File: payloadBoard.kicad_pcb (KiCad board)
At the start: 2 copper layers, 20 x 45 mm, 40 parts, among them J1 USB_C_Receptacle_USB2.0_16P, J2 SERVO, J3 2S Battery, U1 nRF52833_QDxx, U2 AT25SF041-SSHB-X, U3 LSM6DSO32, U4 AP63205WU, U5 AP63203WU, Y2 Crystal_GND24

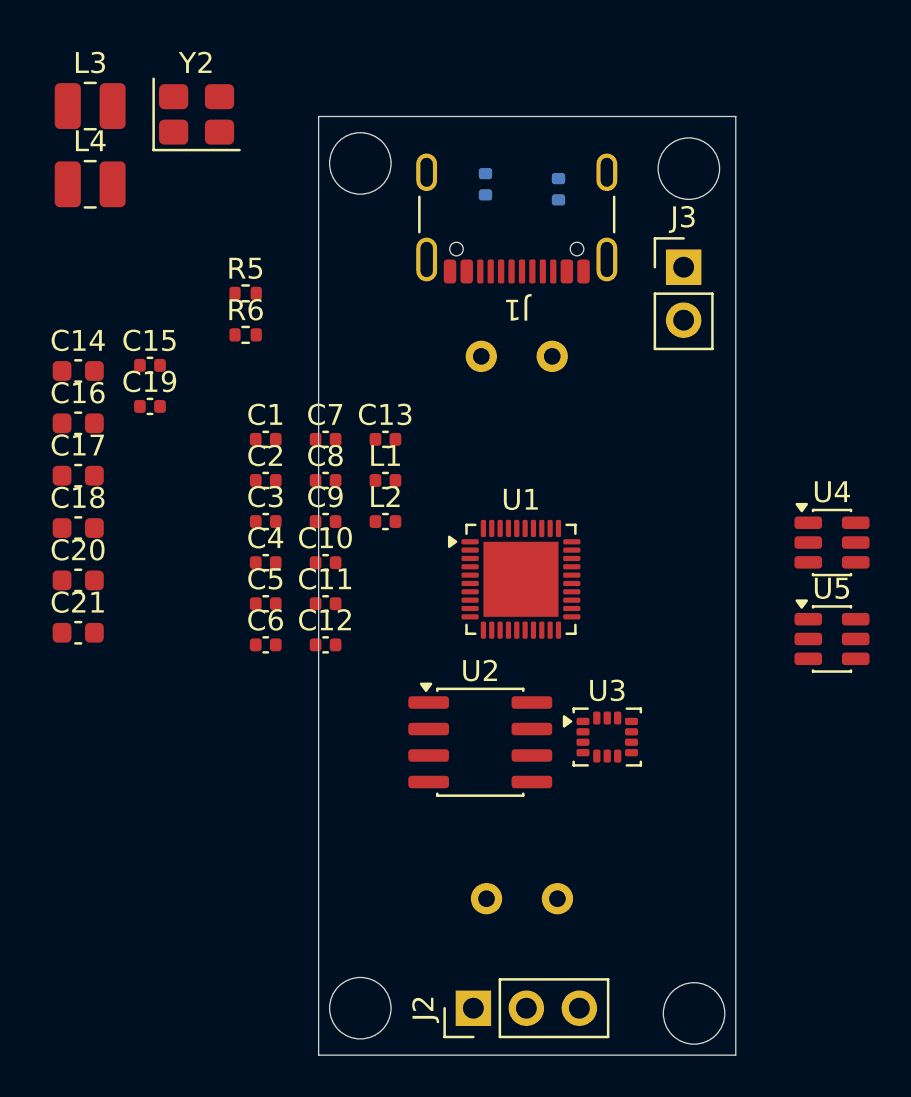
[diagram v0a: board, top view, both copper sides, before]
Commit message: version 1 finished
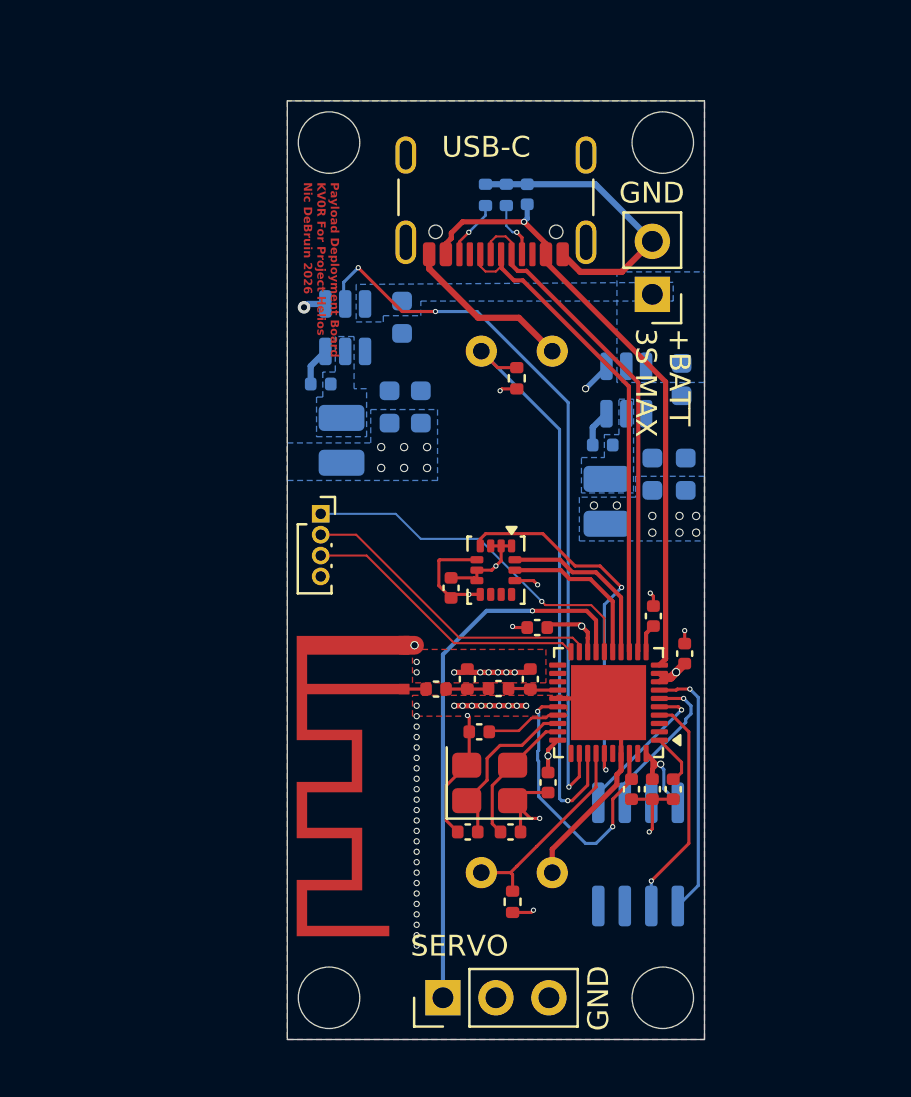
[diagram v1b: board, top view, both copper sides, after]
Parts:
- added AE1: Antenna_Chip, RF_Antenna:Texas_SWRA117D_2.4GHz_Left, F.Cu at (150.6, 93.2)
- added C22: 1uF, Capacitor_SMD:C_0402_1005Metric, F.Cu at (161.5, 98.0)
- added J4: Conn_01x04, Connector_PinSocket_1.00mm:PinSocket_1x04_P1.00mm_Vertical, F.Cu at (146.6, 84.8)
- C14, C15, C16, C17, C18, C19, C20, C21, C7, L3, L4, U2, U4, U5: moved to B.Cu
- moved Y2 35.0 mm to (154.7, 97.7)
- moved R5 31.9 mm to (155.8, 103.4), turned to 90 degrees
- moved C18 29.8 mm to (163.9, 78.4), turned to -90 degrees
- moved C20 29.6 mm to (164.1, 82.9), turned to 90 degrees
- moved L4 29.0 mm to (160.3, 84.2), turned to -90 degrees
- moved C21 28.6 mm to (162.5, 82.9), turned to 90 degrees
- moved R4 26.5 mm to (154.3, 77.0), turned to 0 degrees
- moved U4 25.5 mm to (147.8, 75.9), turned to -90 degrees
- moved R3 25.0 mm to (154.3, 102.0), turned to 0 degrees
- moved C2 24.5 mm to (163.5, 98.0), turned to 90 degrees
- moved C19 21.8 mm to (160.1, 81.5)
- moved L3 20.1 mm to (147.6, 81.3), turned to -90 degrees
- moved C6 18.6 mm to (162.6, 89.7), turned to -90 degrees
- moved C11 18.0 mm to (162.5, 98.0), turned to -90 degrees
- moved C8 18.0 mm to (157.5, 97.7), turned to -90 degrees
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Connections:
- U1 pad 16: unconnected-(U1-P0.18/~{RESET}-Pad16) -> Net-(J4-Pin_1)
- U1 pad 17: unconnected-(U1-P0.20-Pad17) -> PWM
- U1 pad 19: unconnected-(U1-SWDIO-Pad19) -> Net-(J4-Pin_2)
- U1 pad 20: unconnected-(U1-SWDCLK-Pad20) -> Net-(J4-Pin_3)
- U1 pad 32: unconnected-(U1-AIN0/P0.02-Pad32) -> +5V_EN
- U1 pad 35: unconnected-(U1-AIN6/P0.30-Pad35) -> IMU_IRQ1
- U3 pad 4: IMU_IRQ -> IMU_IRQ1
- U4 pad 2: +BATT -> +5V_EN
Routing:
- net GND: track 0.00 -> 64.0 mm, vias 0 -> 49
- net +5V_EN: track 0.00 -> 35.1 mm, vias 0 -> 3
- net VBUS: track 0.00 -> 29.9 mm, vias 0 -> 1
- net ADC0: track 0.00 -> 28.2 mm, vias 0 -> 1
- net PWM: track 0.00 -> 26.4 mm, vias 0 -> 1
- net D-: track 0.00 -> 24.3 mm
- net D+: track 0.00 -> 24.2 mm
- net +3.3V: track 0.00 -> 22.9 mm, vias 0 -> 17
- net IMU_IRQ1: track 0.00 -> 18.2 mm, vias 0 -> 2
- net Net-(J4-Pin_1): track 0.00 -> 17.3 mm, vias 0 -> 1
- net Net-(J4-Pin_2): track 0.00 -> 14.9 mm
- net Net-(U1-DEC4): track 0.00 -> 13.9 mm, vias 0 -> 2
- net Net-(J4-Pin_3): track 0.00 -> 13.9 mm
- net CS: track 0.00 -> 12.5 mm, vias 0 -> 1
- net MISO: track 0.00 -> 10.8 mm, vias 0 -> 1
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- added copper zone on B.Cu, net +3.3V
- added copper zone on In2.Cu, net +3.3V
- added copper zone on B.Cu, net +5V
- added copper zone on In2.Cu, net +5V
- added copper zone on B.Cu, net +BATT
- added copper zone on B.Cu, net GND
- added copper zone on F.Cu, net GND
- added copper zone on In1.Cu, net GND
- added copper zone on B.Cu, net Net-(U4-SW)
- added copper zone on B.Cu, net Net-(U5-SW)
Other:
- outline, holes or cut-outs redrawn
- copper layers 2 -> 4
- board text added: "+BATT 3S MAX"
- board text added: "- 4x #4 Holes absolute max size 60x30mm"
- board text added: "GND"
- board text added: "Payload Deployment Board KV0R For Project Helios Nic DeBruin 2026"
- board text added: "SERVO"
- board text added: "USB-C"
- board text removed: "4x #4 Holes absolute max size 60x30mm"
